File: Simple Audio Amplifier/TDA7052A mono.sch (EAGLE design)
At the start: 16 parts, among them IC1 TDA7052A, IC2 TDA7053A

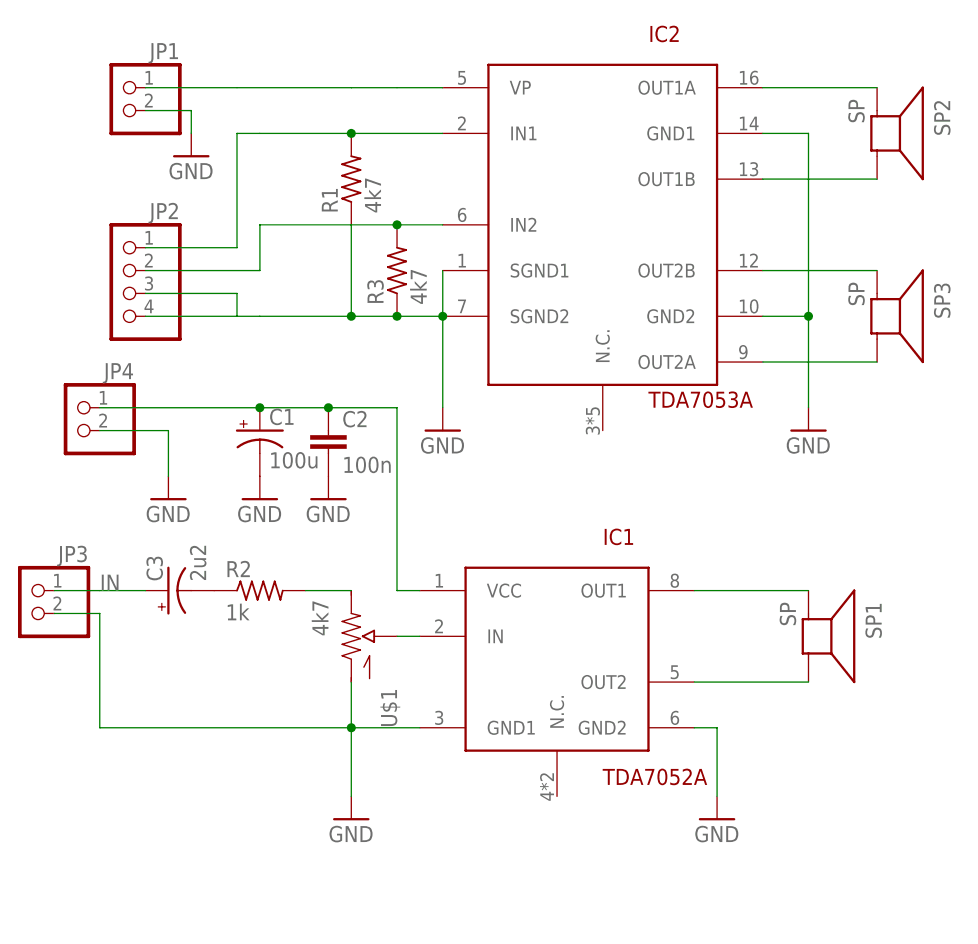
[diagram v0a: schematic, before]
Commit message: Amplifiers
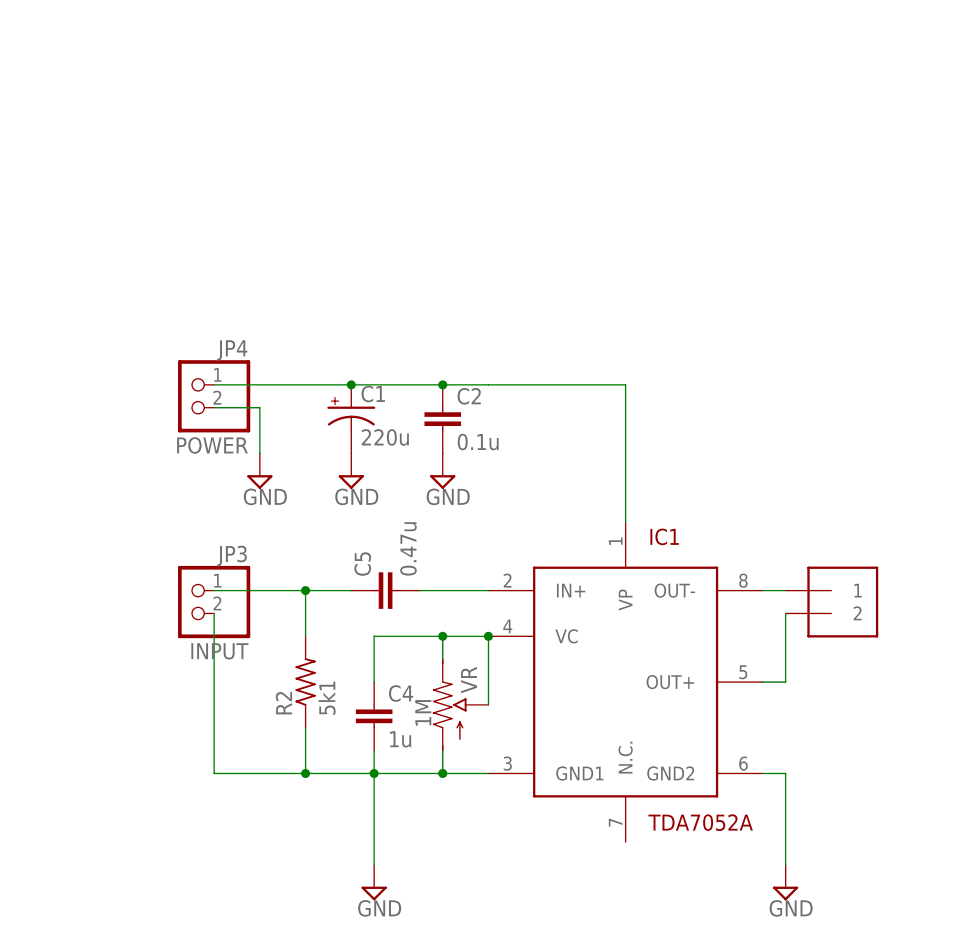
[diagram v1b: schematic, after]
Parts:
- removed C3: 2u2, SparkFun:CAP_POLPTH1
- removed IC2: TDA7053A, My Library:TDA7053A
- removed JP1: (no value), pinhead:PINHD-1X2
- removed JP2: (no value), pinhead:PINHD-1X4
- removed R1, R3: 4k7, adafruit:R-US_0204/5
- removed SP1, SP2, SP3: SP, My Library:SP
- removed U$1: 4k7, My Library:POT-RV16AF-20
- added C4: 1u, SparkFun:CAPPTH2
- added C5: 0.47u, SparkFun:CAPPTH2
- added SPEAKER: 1X2-3.5MM, adafruit:1X2-3.5MM
- added VR: 1M, My Library:POT-RV16AF-20
- C1: value 100u -> 220u
- C2: value 100n -> 0.1u
- JP3: value (none) -> INPUT
- JP4: value (none) -> POWER
- R2: value 1k -> 5k1
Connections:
- removed net IN: C3.+, JP3.1
- removed net N$1: C1.+, C2.1, IC1.VCC, JP4.1
- removed net N$10: IC2.OUT2B, SP3.+
- removed net N$11: IC2.OUT1B, SP2.-
- removed net N$12: IC2.OUT1A, SP2.+
- removed net N$17: IC2.VP, JP1.1
- removed net N$3: R2.2, U$1.E
- removed net N$4: IC2.IN1, JP2.1, R1.2
- removed net N$6: IC2.IN2, JP2.2, R3.2
- removed net N$7: IC2.OUT2A, SP3.-
- new net N$13: C5.1, JP3.1, R2.2
- new net POWER: C1.+, C2.1, IC1.VP, JP4.1
- net GND: now also C4.2, R2.1, VR.A; no longer IC2.GND1, IC2.GND2, IC2.SGND1, IC2.SGND2, JP1.2, JP2.3, JP2.4, R1.1, R3.1, U$1.A
- net N$2: now also C5.2, IC1.IN+; no longer IC1.IN, U$1.S
- net N$5: now also C4.1, IC1.VC, VR.E, VR.S; no longer C3.-, R2.1
- net N$8: now also IC1.OUT-, SPEAKER.1; no longer IC1.OUT1, SP1.+
- net N$9: now also IC1.OUT+, SPEAKER.2; no longer IC1.OUT2, SP1.-
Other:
- moved on the sheet: C1, C2, JP3, JP4, R2
